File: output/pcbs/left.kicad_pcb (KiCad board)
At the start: 2 copper layers, 132.3 x 93.4 mm, 48 parts

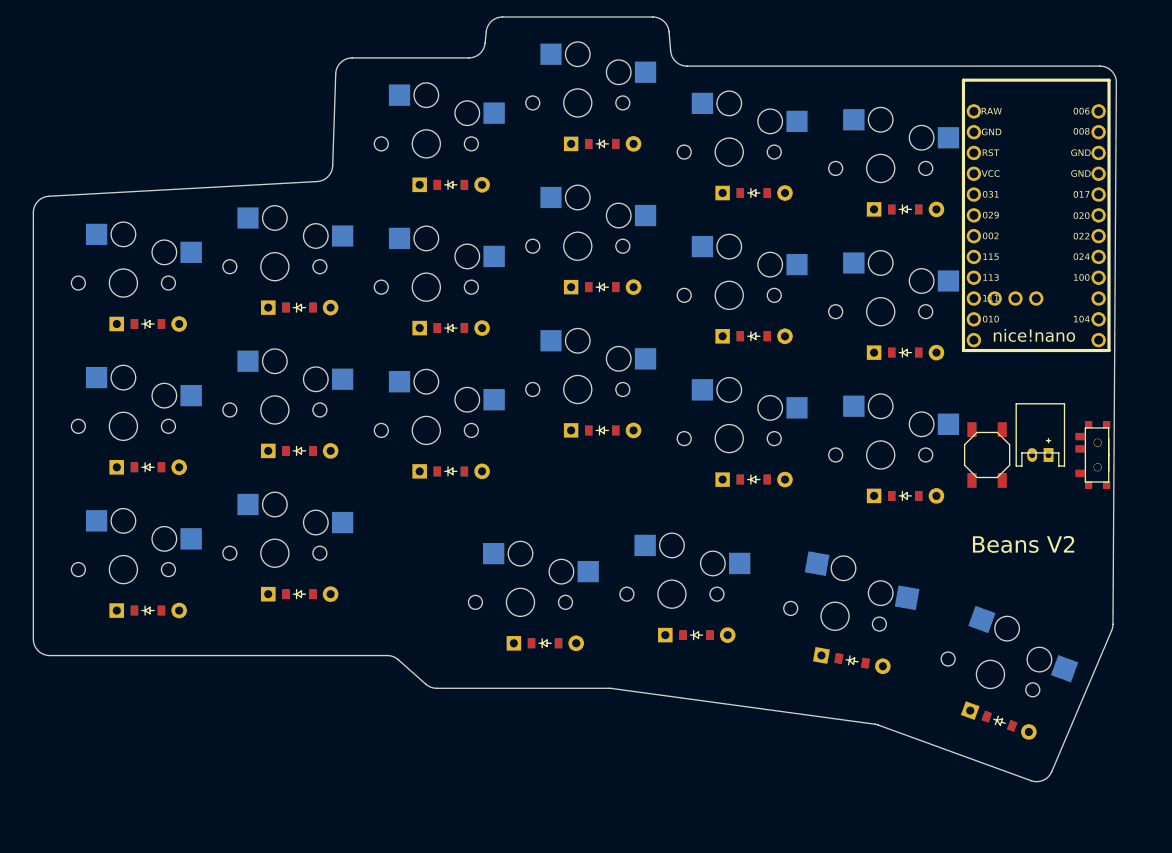
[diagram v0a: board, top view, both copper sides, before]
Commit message: More work on V2
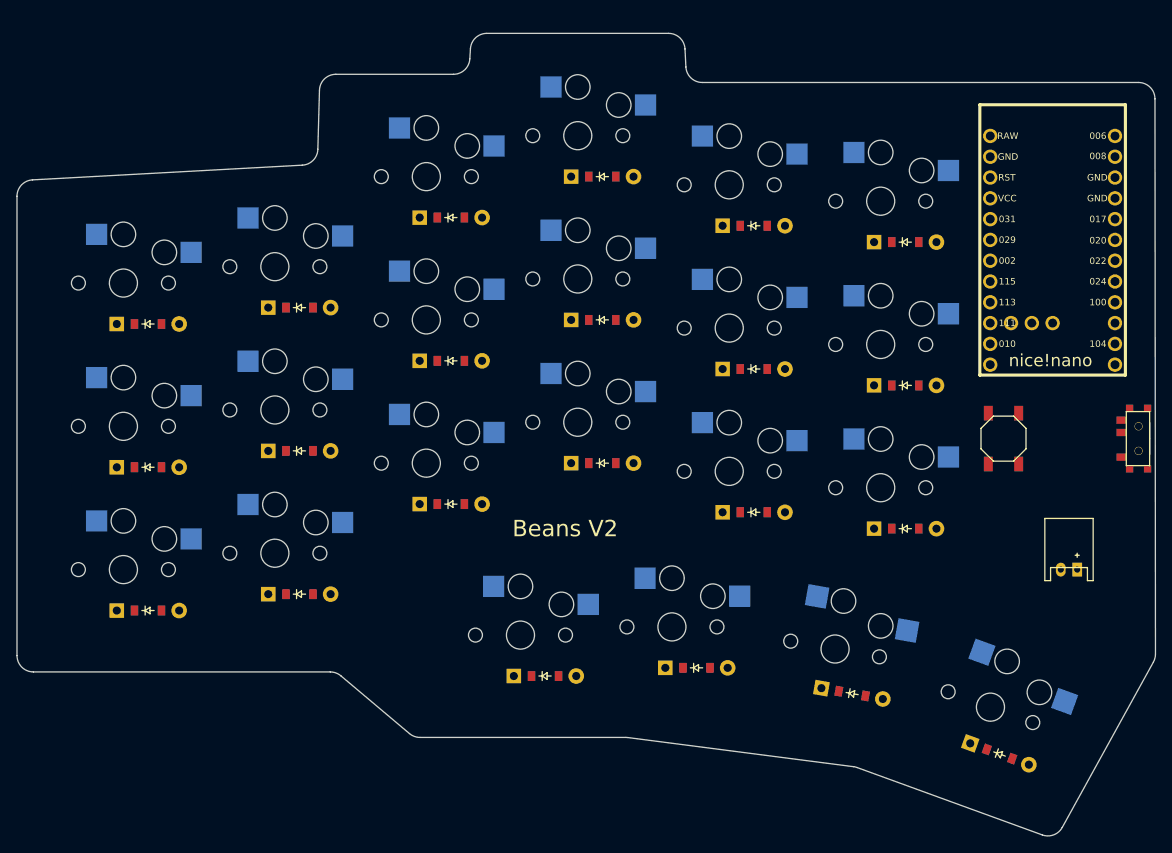
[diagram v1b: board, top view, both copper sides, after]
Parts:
- moved JST1 14.4 mm to (215.5, 82.5)
- moved T1 5.39 mm to (224.0, 66.5)
- moved D10 4.00 mm to (158.5, 69.5)
- moved D11 4.00 mm to (158.5, 52.0)
- moved D12 4.00 mm to (158.5, 34.5)
- moved D13 4.00 mm to (177.0, 75.5)
- moved D14 4.00 mm to (177.0, 58.0)
- moved D15 4.00 mm to (177.0, 40.5)
- moved D16 4.00 mm to (195.5, 77.5)
- moved D17 4.00 mm to (195.5, 60.0)
- moved D18 4.00 mm to (195.5, 42.5)
- moved D19 4.00 mm to (151.5, 95.5)
- moved D20 4.00 mm to (170.0, 94.5)
- moved D21 4.00 mm to (189.0, 97.6)
- moved D22 4.00 mm to (207.0, 105.0)
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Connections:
- S1 pad 1: P031 -> P104
- S10 pad 1: P115 -> P002
- S11 pad 1: P115 -> P002
- S12 pad 1: P115 -> P002
- S13 pad 1: P113 -> P029
- S14 pad 1: P113 -> P029
- S15 pad 1: P113 -> P029
- S16 pad 1: P104 -> P031
- S17 pad 1: P104 -> P031
- S18 pad 1: P104 -> P031
- S19 pad 1: P002 -> P115
- S2 pad 1: P031 -> P104
- S20 pad 1: P115 -> P002
- S21 pad 1: P113 -> P029
- S22 pad 1: P104 -> P031
- S3 pad 1: P031 -> P104
- S4 pad 1: P029 -> P113
- S5 pad 1: P029 -> P113
- S6 pad 1: P029 -> P113
- S7 pad 1: P002 -> P115
- S8 pad 1: P002 -> P115
- S9 pad 1: P002 -> P115
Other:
- board size 132.3 x 93.4 mm -> 139.1 x 98 mm
